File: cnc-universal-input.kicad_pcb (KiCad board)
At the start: 2 copper layers, 96.5 x 96.5 mm, 143 parts, among them J1 3PT, J10 2PT, J12 USB_B_Mini, J13 2PT, J14 2PT, J15 2PT, J16 2PT, J17 2PT, J18 2PT, J2 3PT, J3 3PT, J4 3PT, J5 3PT, J6 3PT, J7 3PT, J8 3PT, J9 AVR-ISP-6, Q1 2N7002, Q11 2N7002, Q12 2N7002, Q13 2N7002, Q2 2N7002, Q3 2N7002, Q4 2N7002, Q5 2N7002, Q6 2N7002, Q7 2N7002, Q8 2N7002, Q9 2N7002, SW1 RESET, SW2 BTN, U1 ATmega328PB-AU, U10 EL357NC, U11 EL357NC, U12 EL357NC, U13 EL357NC, U14 EL357NC, U15 EL357NC, U16 EL357NC, U18 CH340G, U19 XL1509-5E1, U2 74HC595, U3 74HC595, U4 74HC595, U5 4051, U6 XL1509-12E1, U7 ADuM1201AR, U8 SGMOP07CXS8G/TR, U9 EL357NC, Y1 16MHz, Y2 12MHz

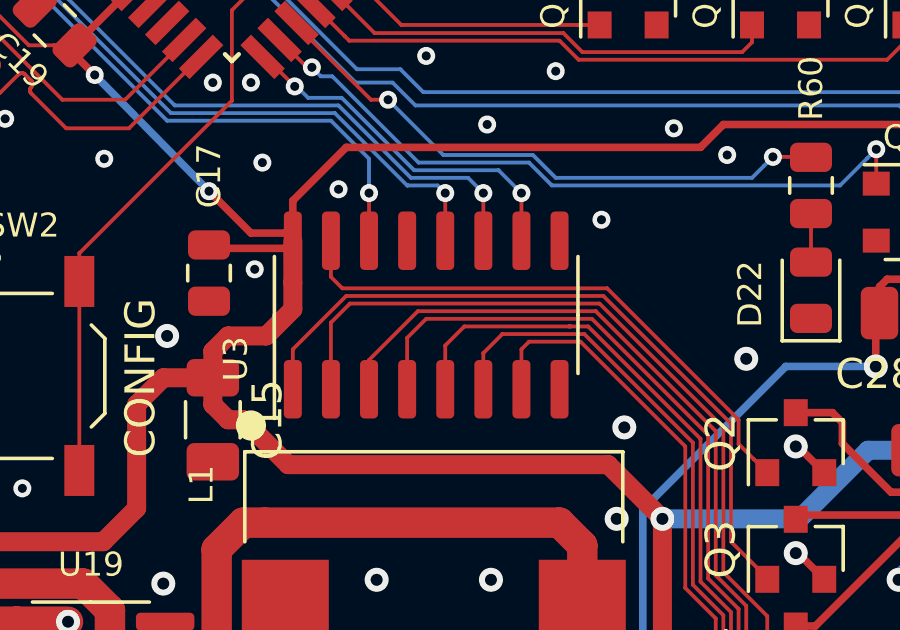
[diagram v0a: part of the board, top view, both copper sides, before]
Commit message: Update cnc-universal-input.kicad_pcb
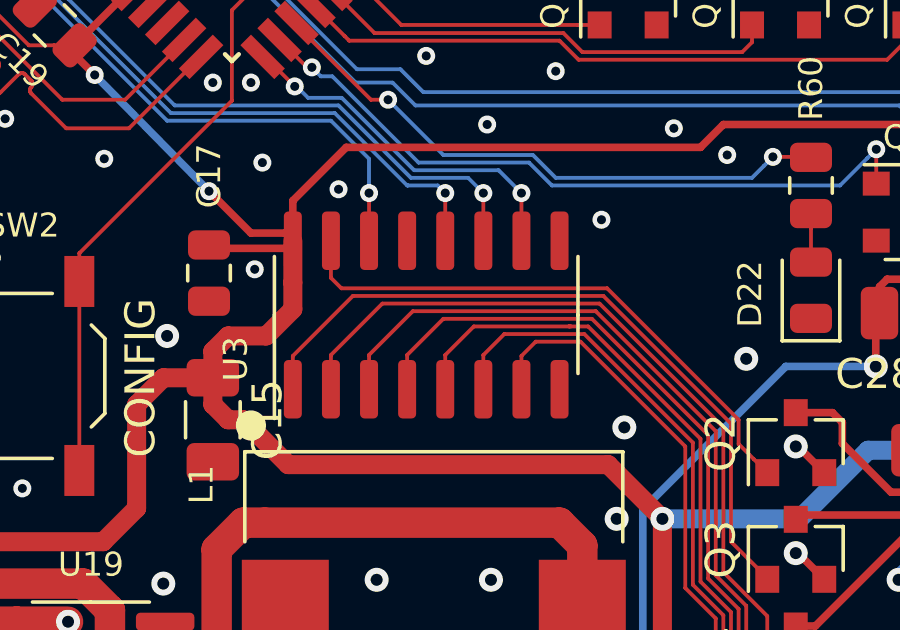
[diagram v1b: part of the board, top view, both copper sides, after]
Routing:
- net /OUT-C: track 26.5 -> 25.9 mm
